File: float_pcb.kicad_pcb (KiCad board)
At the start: 2 copper layers, 68.8 x 41.5 mm, 51 parts, among them J1 BR Switch, J2 5V, J3 USB_C, J5 BR_DEPTH, J6 BR Light, J7 Batt, J8 Conn_01x04, Q1 AO3400A, U1 TPSM863252, U2 TPSM863252, U3 ESP32-S3-MINI-1U

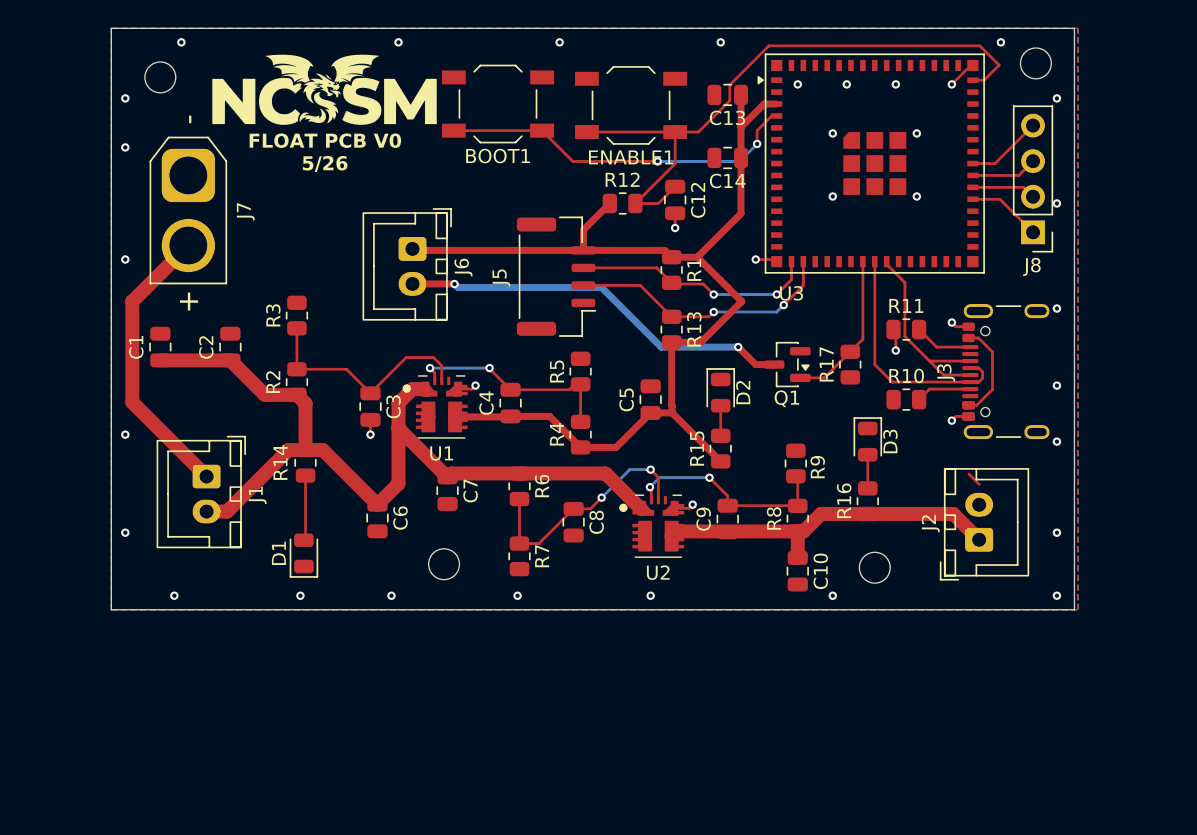
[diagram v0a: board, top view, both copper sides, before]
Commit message: V2
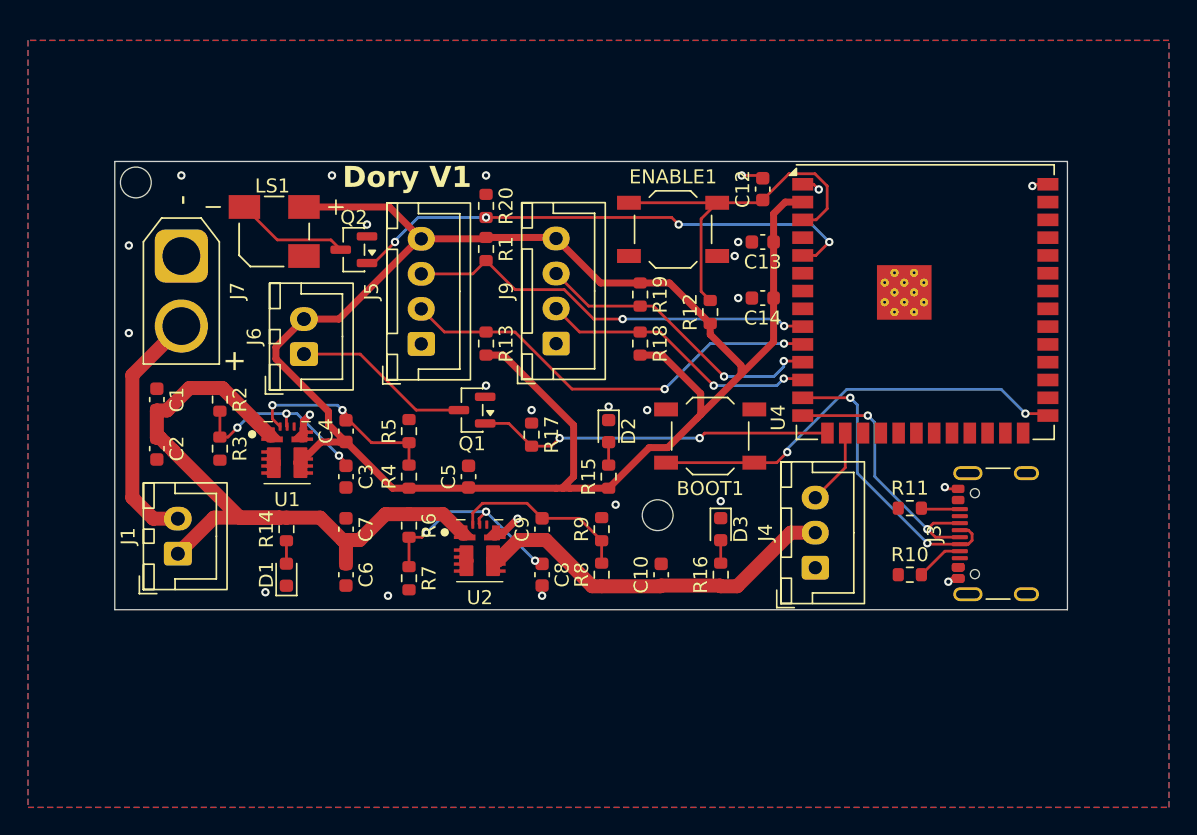
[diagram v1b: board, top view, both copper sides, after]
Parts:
- removed G***: LOGO, LOGO
- removed H3, H4: MH, MountingHole:MountingHole_2.2mm_M2
- removed J2: 5V, Connector_JST:JST_XH_B2B-XH-A_1x02_P2.50mm_Vertical
- removed J8: Conn_01x04, Connector_PinHeader_2.54mm:PinHeader_1x04_P2.54mm_Vertical
- removed U3: ESP32-S3-MINI-1U, RF_Module:ESP32-S2-MINI-1U
- added J4: Conn_01x03, Connector_JST:JST_XH_B3B-XH-A_1x03_P2.50mm_Vertical, F.Cu at (142.2, 100.5)
- added J9: I2C, Connector_JST:JST_XH_B4B-XH-A_1x04_P2.50mm_Vertical, F.Cu at (123.8, 84.5)
- added LS1: SMT-0540-T-9-R, buzzer:XDCR_SMT-0540-T-9-R, F.Cu at (103.6, 76.5)
- added Q2: AO3400A, Package_TO_SOT_SMD:SOT-23, F.Cu at (109.3, 77.8)
- added R18: 4k7, Resistor_SMD:R_0603_1608Metric, F.Cu at (129.8, 84.5)
- added R19: 4k7, Resistor_SMD:R_0603_1608Metric, F.Cu at (129.8, 81.0)
- added R20: 10k, Resistor_SMD:R_0603_1608Metric, F.Cu at (118.8, 74.7)
- added U4: ESP32-S3-WROOM-1, RF_Module:ESP32-S3-WROOM-1U, F.Cu at (150.1, 81.5)
- C1, C10, C12, C13, C14, C2, C3, C4, C5, C6, C7, C8, C9: footprint Capacitor_SMD:C_0805_2012Metric -> Capacitor_SMD:C_0603_1608Metric
- D1: value BATT_STAT -> BATT; footprint LED_SMD:LED_0805_2012Metric -> LED_SMD:LED_0603_1608Metric
- D2: value LED -> 3V3; footprint LED_SMD:LED_0805_2012Metric -> LED_SMD:LED_0603_1608Metric
- D3: value 5V_STAT -> 5V; footprint LED_SMD:LED_0805_2012Metric -> LED_SMD:LED_0603_1608Metric
- J1: value BR Switch -> Switch
- J5: value BR_DEPTH -> I2C; footprint Connector_JST:JST_GH_BM04B-GHS-TBT_1x04-1MP_P1.25mm_Vertical -> Connector_JST:JST_XH_B4B-XH-A_1x04_P2.50mm_Vertical
- J6: value BR Light -> Light
- R1, R10, R11, R12, R13, R14, R15, R16, R17, R2, R3, R4, R5, R6, R7, R8, R9: footprint Resistor_SMD:R_0805_2012Metric -> Resistor_SMD:R_0603_1608Metric
- moved BOOT1 28.1 mm to (134.8, 91.1)
- moved R17 23.3 mm to (122.0, 91.0), turned to -90 degrees
- moved Q1 22.7 mm to (117.8, 89.2)
- moved H2 15.6 mm to (131.0, 96.8), turned to 0 degrees
- moved R9 14.6 mm to (127.0, 97.8)
- moved R8 14.6 mm to (127.0, 101.0)
- moved C5 14.1 mm to (117.5, 94.0)
- moved R1 13.3 mm to (118.8, 77.8)
- moved R13 13.3 mm to (118.8, 84.5)
- moved C9 13.3 mm to (122.8, 97.8)
- moved R5 13.0 mm to (113.2, 90.8)
- moved U2 12.9 mm to (118.3, 99.3)
- moved R11 12.8 mm to (149.0, 96.2)
- moved R4 12.6 mm to (113.2, 94.0)
- moved R10 12.5 mm to (149.0, 101.0)
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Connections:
- net /SCL renamed SCL1
- net /SDA renamed SDA1
- C1 pad 1: +BATT -> GND
- C1 pad 2: GND -> +BATT
- C7 pad 1: +BATT -> GND
- C7 pad 2: GND -> +BATT
- J1 pad 1: Net-(J1-Pin_1) -> +BATT
- J1 pad 2: +BATT -> Net-(J1-Pin_2)
- J6 pad 1: +3V3 -> Net-(J6-Pin_1)
- J6 pad 2: Net-(J6-Pin_2) -> +3V3
- J7 pad 2: Net-(J1-Pin_1) -> Net-(J1-Pin_2)
- Q1 pad 3: Net-(J6-Pin_2) -> Net-(J6-Pin_1)
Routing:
- net +3V3: track 78.9 -> 131.3 mm
- net BUZZER: track 0.00 -> 37.4 mm, vias 0 -> 4
- net Net-(J6-Pin_2): track 28.2 -> 0.00 mm, vias 2 -> 0
- net SCL2: track 0.00 -> 21.4 mm, vias 0 -> 2
- net Net-(J1-Pin_1): track 20.3 -> 0.00 mm
- net SDA2: track 0.00 -> 20.1 mm, vias 0 -> 2
- net Net-(U4-EN): track 45.5 -> 26.8 mm
- net Net-(J1-Pin_2): track 0.00 -> 17.6 mm
- net LIGHT: track 11.1 -> 25.5 mm, vias 0 -> 2
- net Net-(J6-Pin_1): track 0.00 -> 12.7 mm
- net +BATT: track 60.7 -> 48.3 mm
- net SCL1: track 17.4 -> 29.6 mm
- net SDA1: track 19.3 -> 31.0 mm
- net Net-(Q2-D): track 0.00 -> 8.14 mm
- net /USB_VBUS_UNUSED: track 6.96 -> 0.00 mm
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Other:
- board size 68.8 x 41.5 mm -> 68 x 32 mm
- board text added: "Dory V1"
- board text added: "Evan Kim '27"
- board text removed: "FLOAT PCB V0 5/26"

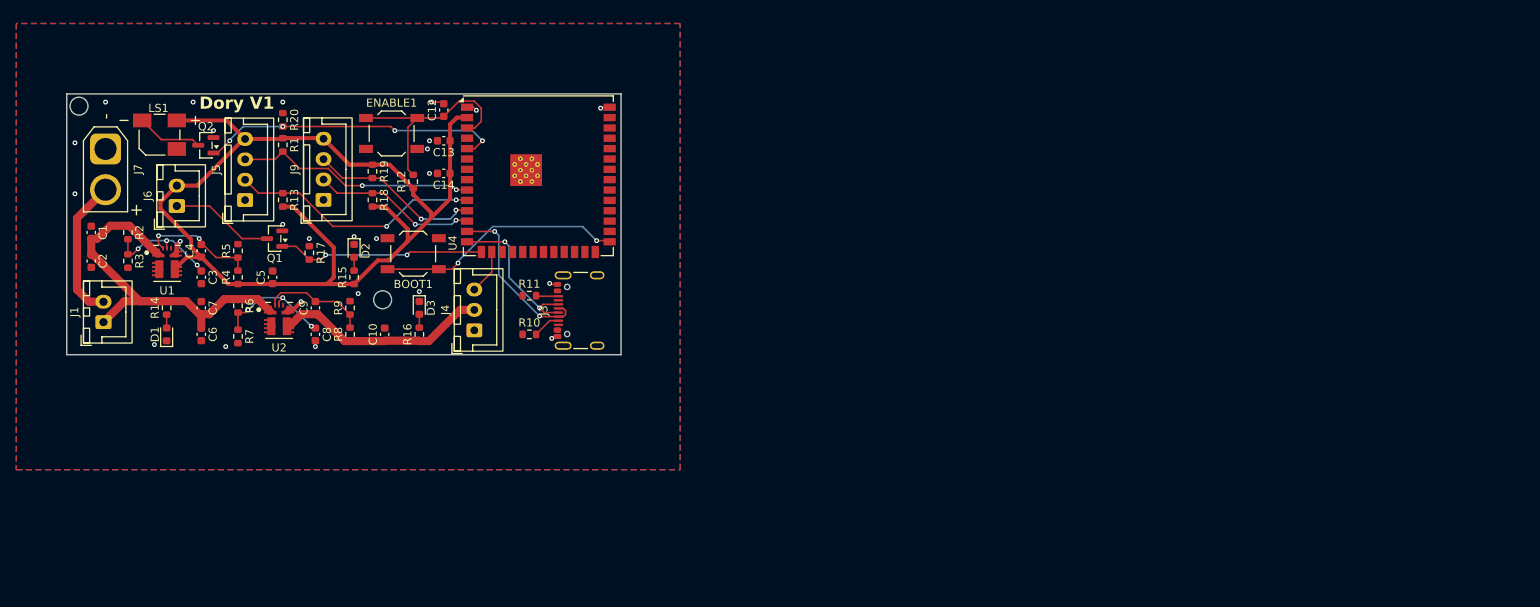
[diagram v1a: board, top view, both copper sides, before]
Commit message: V3
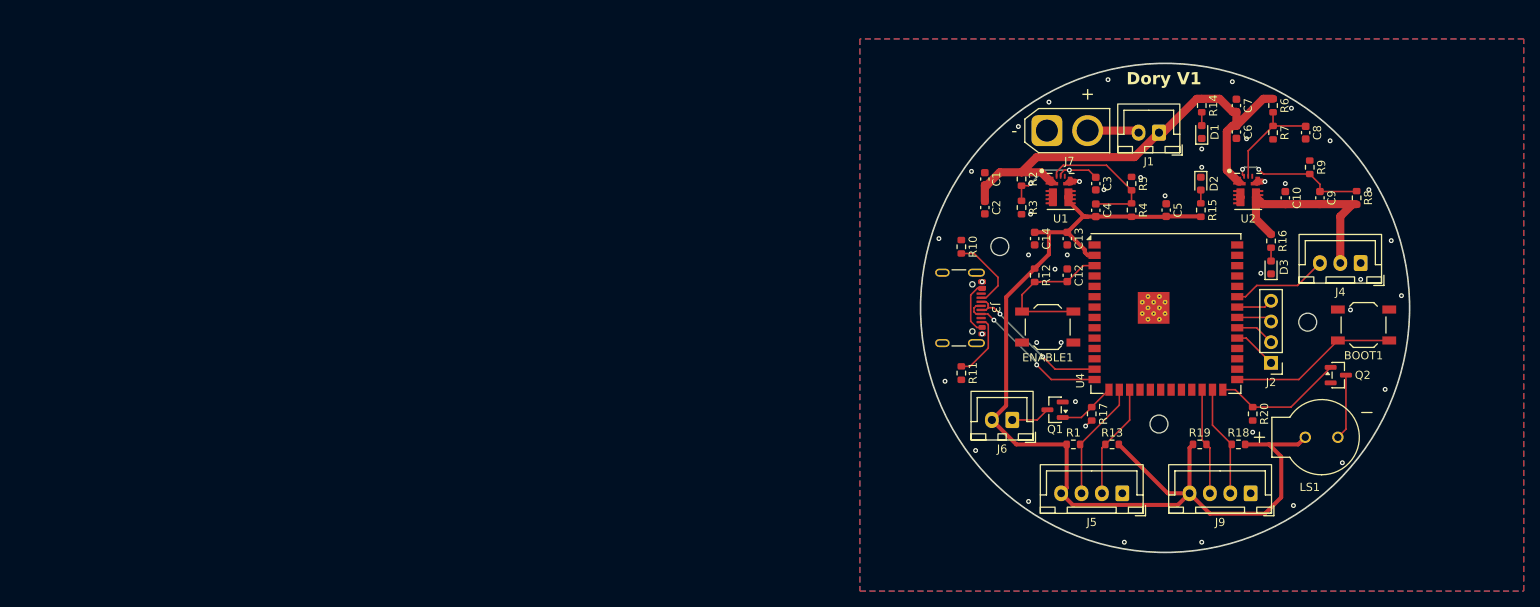
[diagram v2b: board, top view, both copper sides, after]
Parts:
- added H3: MH, MountingHole:MountingHole_2.2mm_M2, F.Cu at (206.7, 90.2)
- added J2: Conn_01x04, Connector_PinHeader_2.54mm:PinHeader_1x04_P2.54mm_Vertical, F.Cu at (240.0, 104.5)
- LS1: value SMT-0540-T-9-R -> AT-1127-ST-2-R; footprint buzzer:XDCR_SMT-0540-T-9-R -> buzzer:XDCR_AT-1127-ST-2-R
- moved LS1 147.3 mm to (246.2, 113.6)
- moved Q2 141.8 mm to (248.2, 106.0), turned to 0 degrees
- moved H1 138.1 mm to (226.2, 112.0)
- moved J1 131.6 mm to (226.2, 76.2), turned to 180 degrees
- moved R7 129.4 mm to (240.2, 76.2)
- moved C6 129.4 mm to (235.8, 76.2)
- moved C7 129.4 mm to (235.8, 72.9)
- moved D1 129.4 mm to (231.5, 76.2)
- moved R14 129.4 mm to (231.5, 72.9), turned to -90 degrees
- moved R6 129.4 mm to (240.2, 72.9)
- moved R8 124.6 mm to (250.5, 84.2), turned to -90 degrees
- moved R20 124.3 mm to (237.8, 110.8)
- moved C8 124.0 mm to (244.2, 76.2)
- moved C9 124.0 mm to (246.0, 84.2), turned to -90 degrees
- moved U2 119.9 mm to (237.2, 83.5)
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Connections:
- C10 pad 1: Net-(J4-Pin_2) -> GND
- C10 pad 2: GND -> Net-(J4-Pin_2)
- C12 pad 1: Net-(U4-EN) -> GND
- C12 pad 2: GND -> Net-(U4-EN)
- C4 pad 1: +3V3 -> Net-(U1-FB)
- C4 pad 2: Net-(U1-FB) -> +3V3
- C5 pad 1: +3V3 -> GND
- C5 pad 2: GND -> +3V3
- C9 pad 1: Net-(J4-Pin_2) -> Net-(U2-FB)
- C9 pad 2: Net-(U2-FB) -> Net-(J4-Pin_2)
- ENABLE1 pad 1: Net-(U4-EN) -> GND
- ENABLE1 pad 2: GND -> Net-(U4-EN)
- R11 pad 1: GND -> Net-(J3-CC2)
- R11 pad 2: Net-(J3-CC2) -> GND
- R14 pad 1: Net-(D1-A) -> +BATT
- R14 pad 2: +BATT -> Net-(D1-A)
- R15 pad 1: +3V3 -> Net-(D2-A)
- R15 pad 2: Net-(D2-A) -> +3V3
- R17 pad 1: GND -> LIGHT
- R17 pad 2: LIGHT -> GND
- R20 pad 1: GND -> BUZZER
- R20 pad 2: BUZZER -> GND
- R4 pad 1: +3V3 -> Net-(U1-FB)
- R4 pad 2: Net-(U1-FB) -> +3V3
- R5 pad 1: Net-(U1-FB) -> GND
- R5 pad 2: GND -> Net-(U1-FB)
- R8 pad 1: Net-(J4-Pin_2) -> Net-(U2-FB)
- R8 pad 2: Net-(U2-FB) -> Net-(J4-Pin_2)
- R9 pad 1: Net-(U2-FB) -> GND
- R9 pad 2: GND -> Net-(U2-FB)
- U4 pad 10: SDA1 -> unconnected-(U4-IO17-Pad10)
- U4 pad 11: SCL2 -> unconnected-(U4-IO18-Pad11)
- U4 pad 12: SDA2 -> unconnected-(U4-IO8-Pad12)
- U4 pad 16: SERVO -> SCL1
- U4 pad 17: unconnected-(U4-IO9-Pad17) -> SDA1
- U4 pad 24: unconnected-(U4-IO47-Pad24) -> SCL2
- U4 pad 25: unconnected-(U4-IO48-Pad25) -> SDA2
- U4 pad 26: unconnected-(U4-IO45-Pad26) -> BUZZER
- U4 pad 31: unconnected-(U4-IO38-Pad31) -> Net-(J2-Pin_1)
- U4 pad 32: unconnected-(U4-IO39-Pad32) -> Net-(J2-Pin_2)
- U4 pad 33: unconnected-(U4-IO40-Pad33) -> Net-(J2-Pin_3)
- U4 pad 34: unconnected-(U4-IO41-Pad34) -> Net-(J2-Pin_4)
- U4 pad 35: unconnected-(U4-IO42-Pad35) -> SERVO
- U4 pad 5: BUZZER -> unconnected-(U4-IO5-Pad5)
- U4 pad 9: SCL1 -> unconnected-(U4-IO16-Pad9)
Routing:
- net BUZZER: track 37.4 -> 16.1 mm, vias 4 -> 0
- net LIGHT: track 25.5 -> 7.10 mm, vias 2 -> 0
- net SDA1: track 31.0 -> 14.1 mm, vias 2 -> 0
- net SCL1: track 29.6 -> 14.8 mm, vias 2 -> 0
- net Net-(J1-Pin_2): track 17.6 -> 6.35 mm
- net Net-(U4-IO0): track 30.3 -> 20.6 mm, vias 2 -> 0
- net +BATT: track 48.3 -> 57.7 mm
- net SCL2: track 21.4 -> 13.1 mm, vias 2 -> 0
- net Net-(U4-EN): track 26.8 -> 18.7 mm
- net Net-(J6-Pin_1): track 12.7 -> 4.83 mm
- net /USB_VBUS_UNUSED: track 0.00 -> 6.68 mm
- net SDA2: track 20.1 -> 13.8 mm, vias 2 -> 0
- net SERVO: track 5.50 -> 11.9 mm
- net GND: track 9.41 -> 3.12 mm, vias 25 -> 42
- net Net-(J3-CC1): track 3.44 -> 9.42 mm
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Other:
- board size 68 x 32 mm -> 60 x 60 mm
- board text removed: "Evan Kim '27"
